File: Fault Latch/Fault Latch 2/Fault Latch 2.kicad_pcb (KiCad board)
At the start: 2 copper layers, 85 x 85 mm, 108 parts, among them J1 1053141312, J3 1053131202, J4 1053131202, K3 Fujitsu_FTR-LYCA005x, K5 Fujitsu_FTR-LYCA005x, K6 Fujitsu_FTR-LYCA005x, Q101 Q_NPN_BEC, Q102 Q_NPN_BEC, Q103 Q_NPN_BEC, Q104 Q_NPN_BEC, Q105 Q_NMOS_GSD, Q106 Q_NMOS_GSD, Q110 Q_NPN_BEC, Q111 Q_NPN_BEC, Q112 Q_NMOS_GSD, Q113 Q_NMOS_GSD, Q114 Q_NMOS_GSD, Q115 Q_NMOS_GSD, Q117 Q_NMOS_GSD, Q118 Q_NMOS_GSD, Q119 Q_NMOS_GSD, Q120 Q_NMOS_GSD, Q121 Q_NMOS_GSD, Q122 Q_NMOS_GSD, SW101 SW_Omron_B3FS, SW102 SW_Omron_B3FS, SW103 SW_Omron_B3FS, U1 74LS279, U104 74AHC1G00, U109 74AHC1G00, U112 74AHC1G00, U117 74AHC1G00, U118 LM555xM, U2 LM1117DT-5.0, U7 SN74AHC1G08DBVR, U8 SN74AHC1G08DBVR

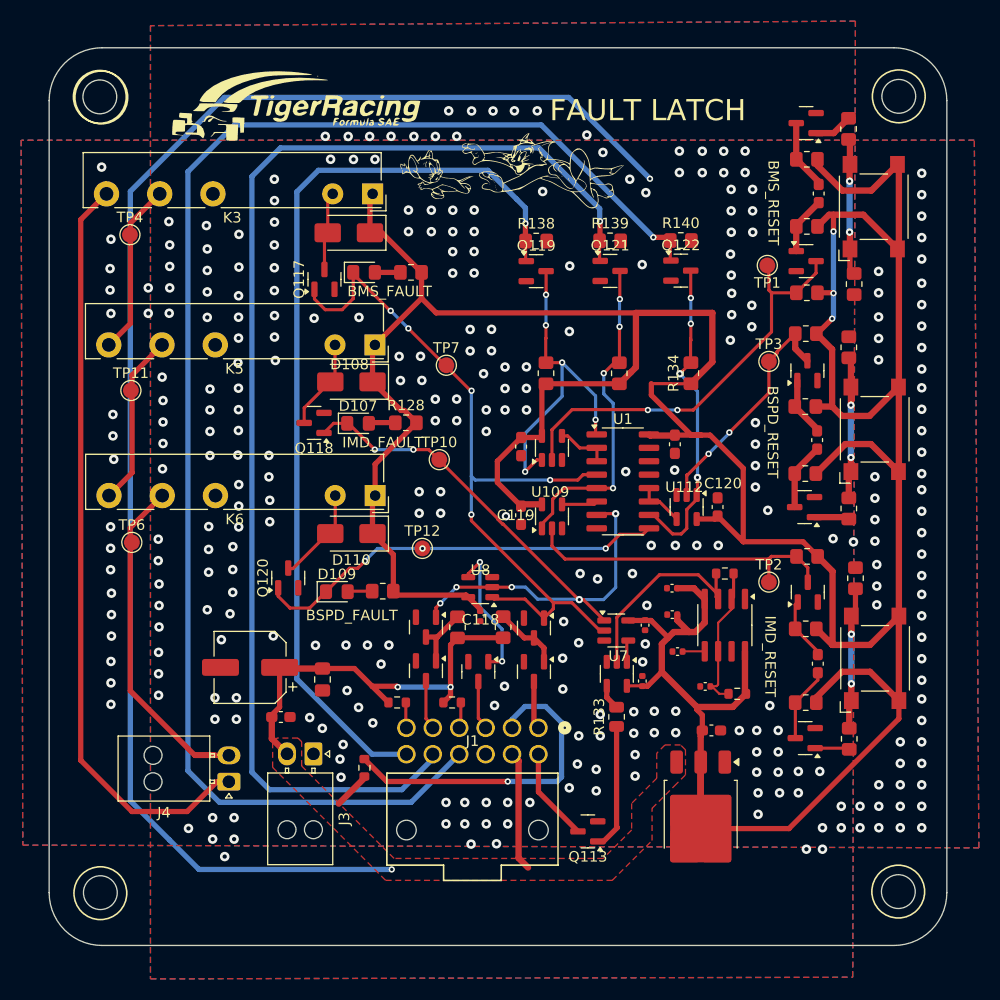
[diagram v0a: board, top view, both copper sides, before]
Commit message: Fault Latch V3
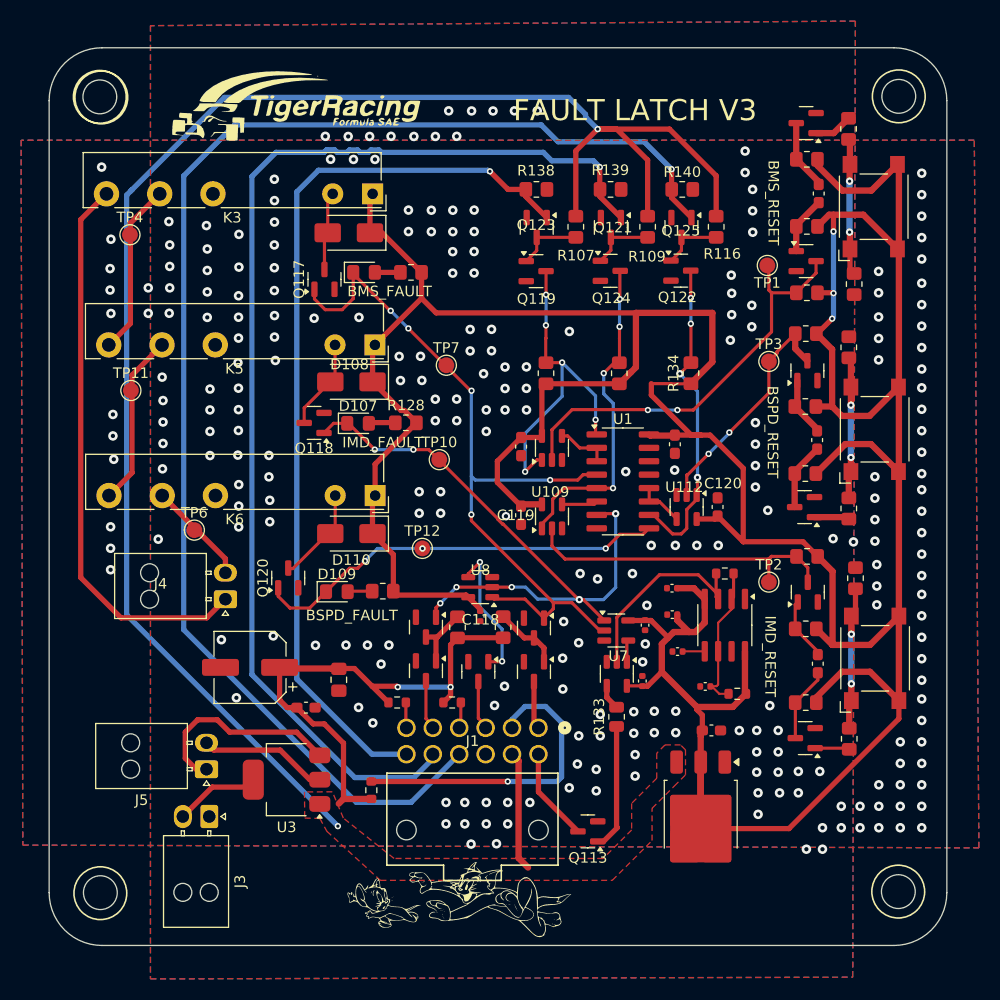
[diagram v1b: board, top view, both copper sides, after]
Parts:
- added J5: 1053131202, Connector_Molex:Molex_Nano-Fit_105313-xx02_1x02_P2.50mm_Horizontal, F.Cu at (84.2, 112.7)
- added Q123: Q_NMOS_GSD, Package_TO_SOT_SMD:SOT-23, F.Cu at (115.4, 61.4)
- added Q124: Q_NMOS_GSD, Package_TO_SOT_SMD:SOT-23, F.Cu at (122.5, 61.4)
- added Q125: Q_NMOS_GSD, Package_TO_SOT_SMD:SOT-23, F.Cu at (129.2, 61.4)
- added R107: 1k, Resistor_SMD:R_0805_2012Metric_Pad1.20x1.40mm_HandSolder, F.Cu at (119.2, 61.3)
- added R109: 1k, Resistor_SMD:R_0805_2012Metric_Pad1.20x1.40mm_HandSolder, F.Cu at (126.0, 61.3)
- added R116: 1k, Resistor_SMD:R_0805_2012Metric_Pad1.20x1.40mm_HandSolder, F.Cu at (132.4, 61.3)
- added U3: ~, Package_TO_SOT_SMD:SOT-223, F.Cu at (91.8, 113.7)
- moved G*** 69.2 mm to (107.3, 124.9)
- moved J4 17.3 mm to (86.0, 96.6)
- moved J3 11.5 mm to (84.4, 117.2)
- moved TP6 6.03 mm to (83.0, 90.0)
- moved R138 4.89 mm to (115.4, 57.8)
- moved R139 4.87 mm to (122.4, 57.8)
- moved R140 4.84 mm to (129.2, 57.8)
- moved C115 2.54 mm to (93.6, 106.9)
- moved R135 2.23 mm to (99.8, 114.7)
- moved C114 1.55 mm to (96.7, 104.2)
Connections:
- J3 pad 2: +12V -> /LVB
- Q119 pad 1: /NBMS_HV -> Net-(Q119-G)
- Q121 pad 1: /IMD_HV -> Net-(Q121-G)
- Q122 pad 1: /BSPD_HV -> Net-(Q122-G)
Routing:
- net /Shutdown Circuit Out: track 33.5 -> 9.79 mm
- net +12V: track 195.0 -> 216.1 mm
- net /Load Switch +: track 0.00 -> 19.5 mm
- net /Shutdown Circuit In: track 71.9 -> 53.4 mm
- net /Load Switch -: track 0.00 -> 12.2 mm
- net /LVB: track 0.00 -> 8.12 mm
- net /IMD_HV: track 117.0 -> 109.7 mm
- net /BSPD_HV: track 139.5 -> 133.0 mm
- net Net-(Q119-G): track 0.00 -> 6.36 mm
- net Net-(Q121-G): track 0.00 -> 6.11 mm
- net Net-(Q122-G): track 0.00 -> 5.92 mm
- net /NBMS_HV: track 88.5 -> 86.2 mm
- net /BMS Light In: track 31.5 -> 30.0 mm
- net GND: vias 313 -> 260
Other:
- board text added: "FAULT LATCH V3"
- board text removed: "FAULT LATCH"
